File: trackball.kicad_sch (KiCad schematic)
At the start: 196 parts, among them J1 ZX-PM2.0-2-4PY, Q1 SI2302_C2891732, SW1 HX TC-5608-Y, SW2 HX TC-5608-Y, SW3 HX TC-5608-Y, SW4 HX TC-5608-Y, SW5 HX TC-5608-Y, SW6 HX TC-5608-Y, SW7 HX TC-5608-Y, SW8 HX TC-5608-Y, U1 SY8089A1AAC, U10 WS2812B, U11 WS2812B, U12 WS2812B, U13 WS2812B, U14 WS2812B, U15 WS2812B, U16 WS2812B, U17 WS2812B, U18 WS2812B, U19 WS2812B, U2 USB-TYPE-C-017, U20 WS2812B, U21 ANT3216LL00R2400A, U3 PMW3610, U4 PMW3610, U5 WS2812B, U6 WS2812B, U7 WS2812B, U8 WS2812B, U9 WS2812B, X1 XL7EL89CKI-111YLC-32M

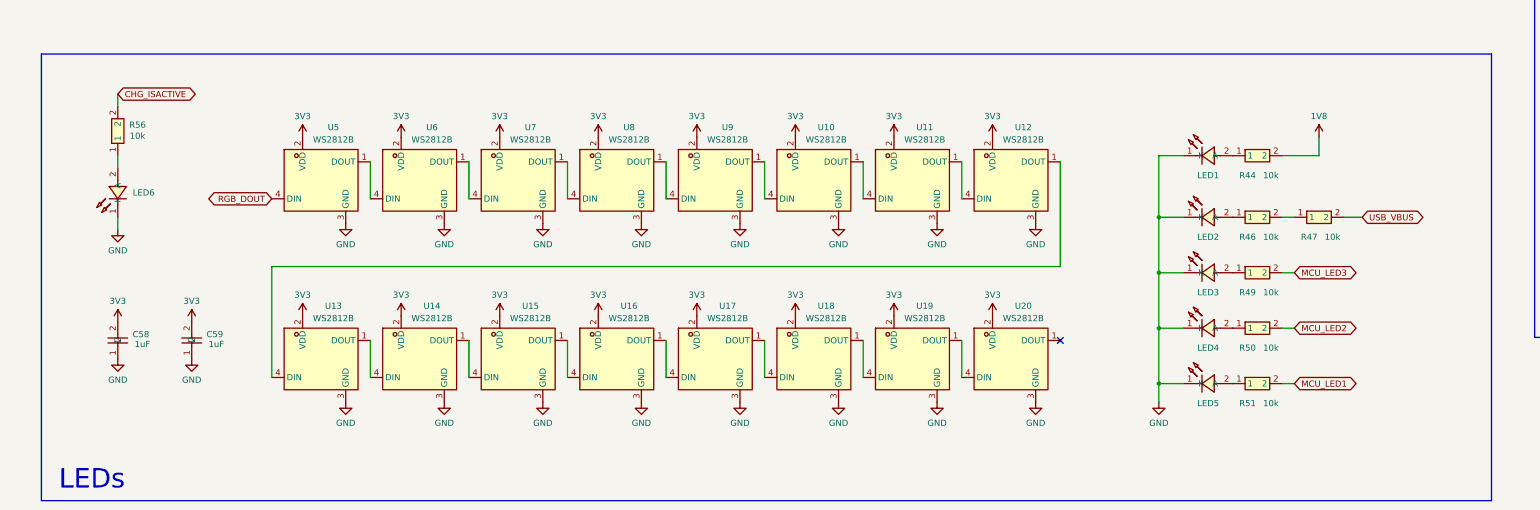
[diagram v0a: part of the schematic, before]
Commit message: chore: checkpoint
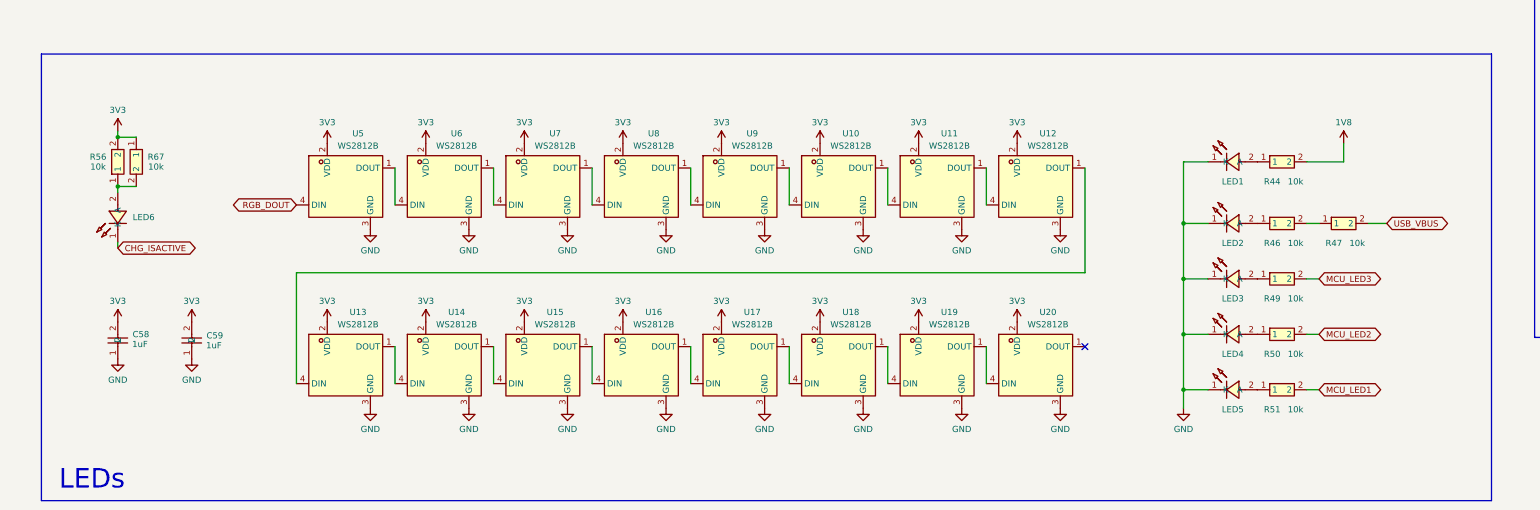
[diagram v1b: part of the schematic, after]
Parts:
- added R67: FRC0402F1002TS, easyeda2kicad:R0402, symbol easyeda2kicad:FRC0402F1002TS
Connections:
- net 3V3: now also R56.2, R67.1
- net CHG_ISACTIVE: now also LED6.1 (K); no longer R56.2
- net GND: no longer LED6.1 (K)
- net at LED6.2 (A), R56.1: now also R67.2
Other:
- moved on the sheet: LED1, LED2, LED3, LED4, LED5, LED6, R44, R46, R47, R49, R50, R51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
